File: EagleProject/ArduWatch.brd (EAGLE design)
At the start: 35.5 x 42.9 mm, 23 parts, among them IC1 DS1307Z, IC2 MCP73831, J1 FTS-105-01-L-D, Q1 32.768Hz, U1 ATMEGA328P_TQFP

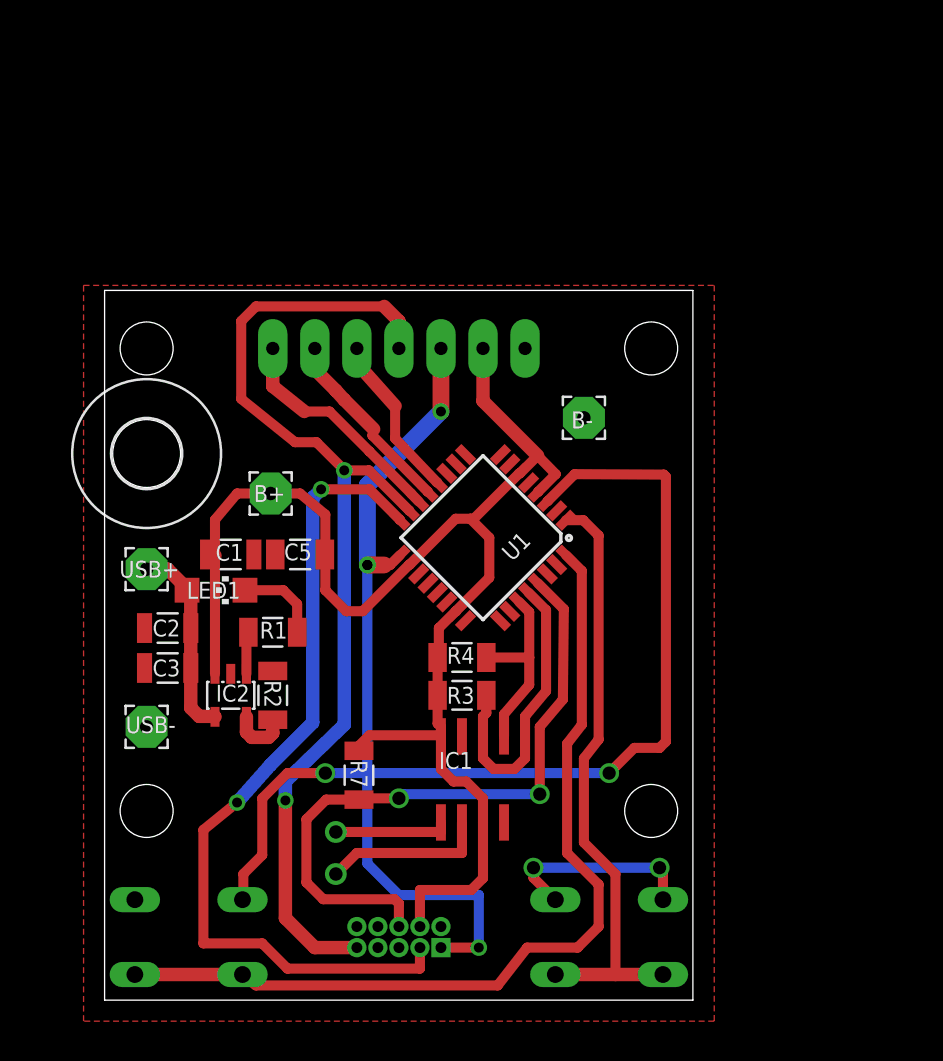
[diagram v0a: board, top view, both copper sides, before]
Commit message: PCB release
PCB release
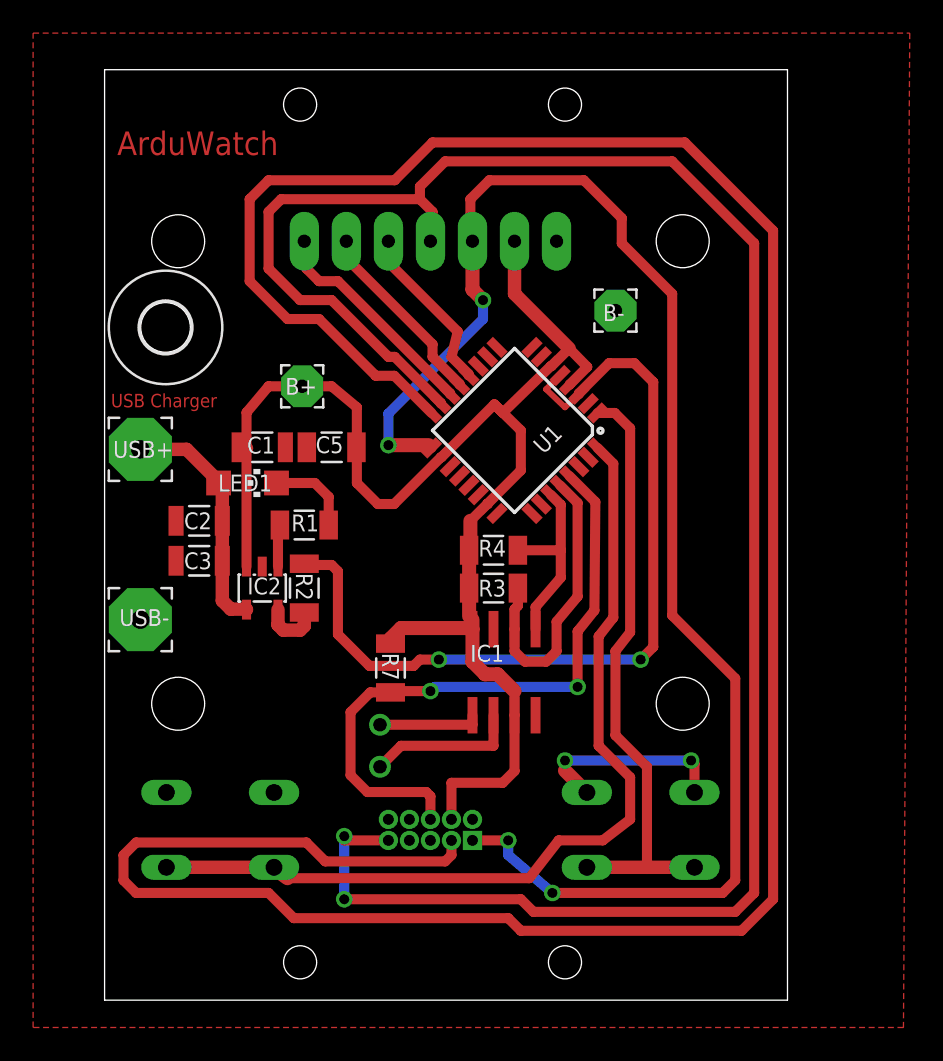
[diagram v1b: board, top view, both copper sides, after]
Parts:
- added DRILEGEND: (no value), drilegend:DRILEGEND
- H5: value MOUNT-HOLE4.1 -> MOUNT-HOLE3.0; device holes:4,1 -> holes:3,0
- USB+, USB-: value WIREPAD2,54/0,8 -> WIREPAD3,81/1,1; device wirepad:2,54/0,8 -> wirepad:3,81/1,1
- moved H5 7.71 mm to (3.68, 40.6)
- moved USB+ 7.25 mm to (2.16, 33.3)
- moved Q1 7.00 mm to (16.6, 15.4)
- moved B+ 6.75 mm to (11.9, 37.1)
- moved C1 6.75 mm to (9.53, 33.4)
- moved C5 6.75 mm to (13.7, 33.4)
- moved C2 6.75 mm to (5.71, 29.0)
- moved C3 6.75 mm to (5.71, 26.5)
- moved IC2 6.75 mm to (9.53, 24.9)
- moved J1 6.75 mm to (17.1, 10.9)
- moved LED1 6.75 mm to (8.64, 31.2)
- moved R1 6.75 mm to (12.1, 28.7)
- moved R2 6.75 mm to (12.1, 24.9)
- moved R3 6.75 mm to (23.5, 24.9)
- moved R4 6.75 mm to (23.5, 27.2)
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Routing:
- net D12: track 51.0 -> 159.3 mm, vias 2 -> 0
- net D11: track 63.0 -> 124.8 mm
- net D13: track 48.2 -> 91.6 mm
- net GND: track 68.4 -> 64.2 mm
- net VUSB: track 12.2 -> 14.8 mm
- net RESET: track 40.0 -> 38.7 mm
- net VCC: track 88.1 -> 89.2 mm
- net N$2: track 6.92 -> 6.16 mm
- net N$5: track 9.99 -> 9.23 mm
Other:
- board size 35.5 x 42.9 mm -> 41.3 x 56.2 mm
- board text added: "ArduWatch"
- board text added: "USB Charger"
